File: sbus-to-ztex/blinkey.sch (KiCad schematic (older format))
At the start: 16 parts

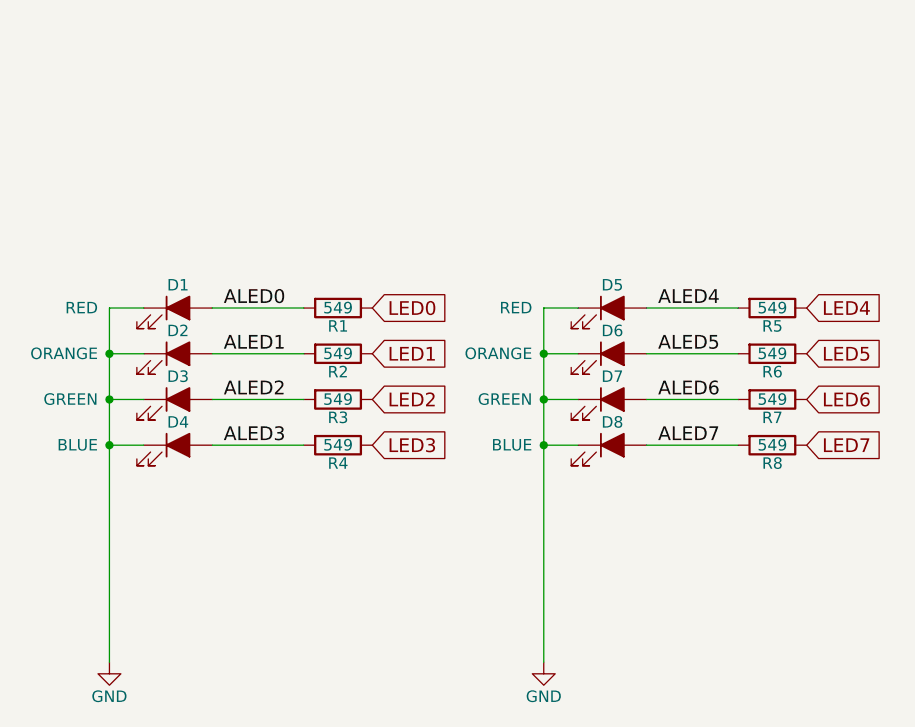
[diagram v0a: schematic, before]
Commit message: Commit first go at v1.2
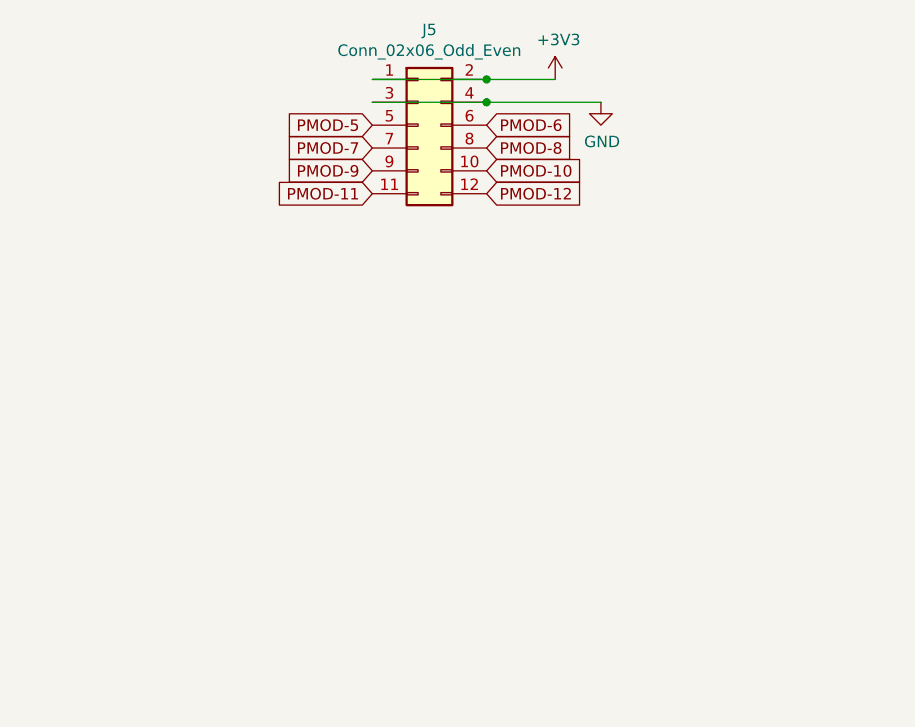
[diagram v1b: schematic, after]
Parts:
- removed D1, D5: RED, LED_SMD:LED_0805_2012Metric, symbol Device:LED_ALT
- removed D2, D6: ORANGE, LED_SMD:LED_0805_2012Metric, symbol Device:LED_ALT
- removed D3, D7: GREEN, LED_SMD:LED_0805_2012Metric, symbol Device:LED_ALT
- removed D4, D8: BLUE, LED_SMD:LED_0805_2012Metric, symbol Device:LED_ALT
- removed R1, R2, R3, R4, R5, R6, R7, R8: 549, Resistor_SMD:R_0603_1608Metric, symbol Device:R
- added J5: Conn_02x06_Odd_Even, Connector_PinSocket_2.54mm:PinSocket_2x06_P2.54mm_Horizontal, symbol Connector_Generic:Conn_02x06_Odd_Even
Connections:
- net GND: now also J5.3 (Pin_3), J5.4 (Pin_4)
- new net +3V3: J5.1 (Pin_1), J5.2 (Pin_2)
- new net PMOD-10: J5.10 (Pin_10)
- new net PMOD-11: J5.11 (Pin_11)
- new net PMOD-12: J5.12 (Pin_12)
- new net PMOD-5: J5.5 (Pin_5)
- new net PMOD-6: J5.6 (Pin_6)
- new net PMOD-7: J5.7 (Pin_7)
- new net PMOD-8: J5.8 (Pin_8)
- new net PMOD-9: J5.9 (Pin_9)
